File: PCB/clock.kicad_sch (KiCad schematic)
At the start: 22 parts, among them J1 USB_C_Receptacle, J2 Conn_01x08, J3 Conn_01x02_Pin, J4 Conn_01x05, J5 Conn_01x05, J6 Conn_01x08, J7 Conn_01x02_Pin, J8 Conn_01x05, J9 Conn_01x05, SW1 RotaryEncoder_Switch_MP, SW2 RotaryEncoder_Switch_MP, U1 ESP32-S3-MINI-1, U2 AMS1117-3.3

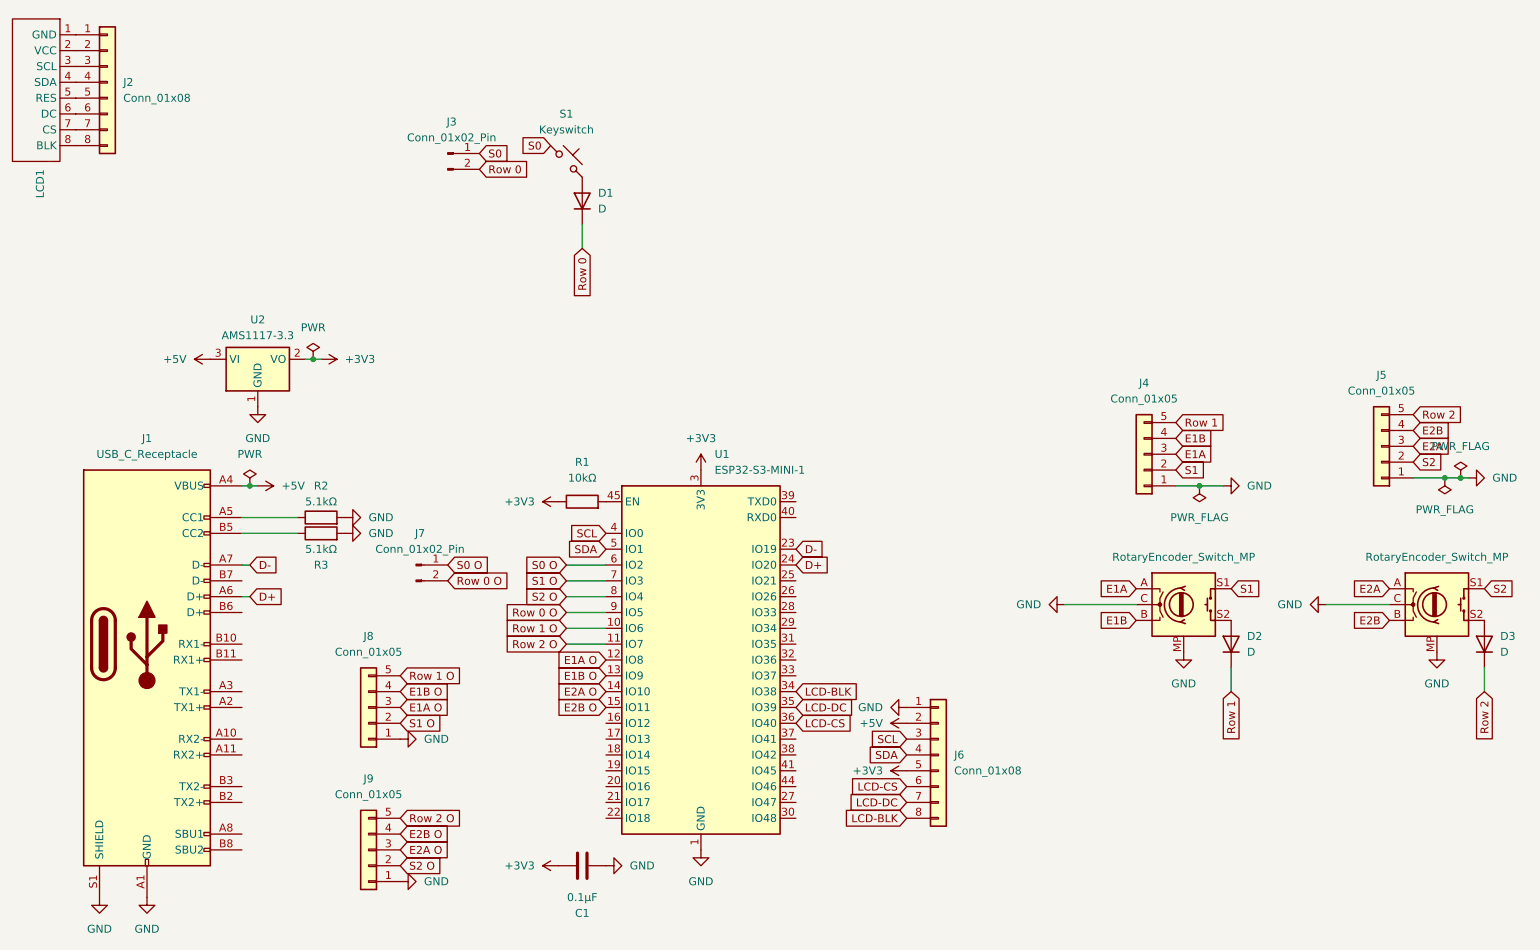
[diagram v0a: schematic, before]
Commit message: Add files via upload
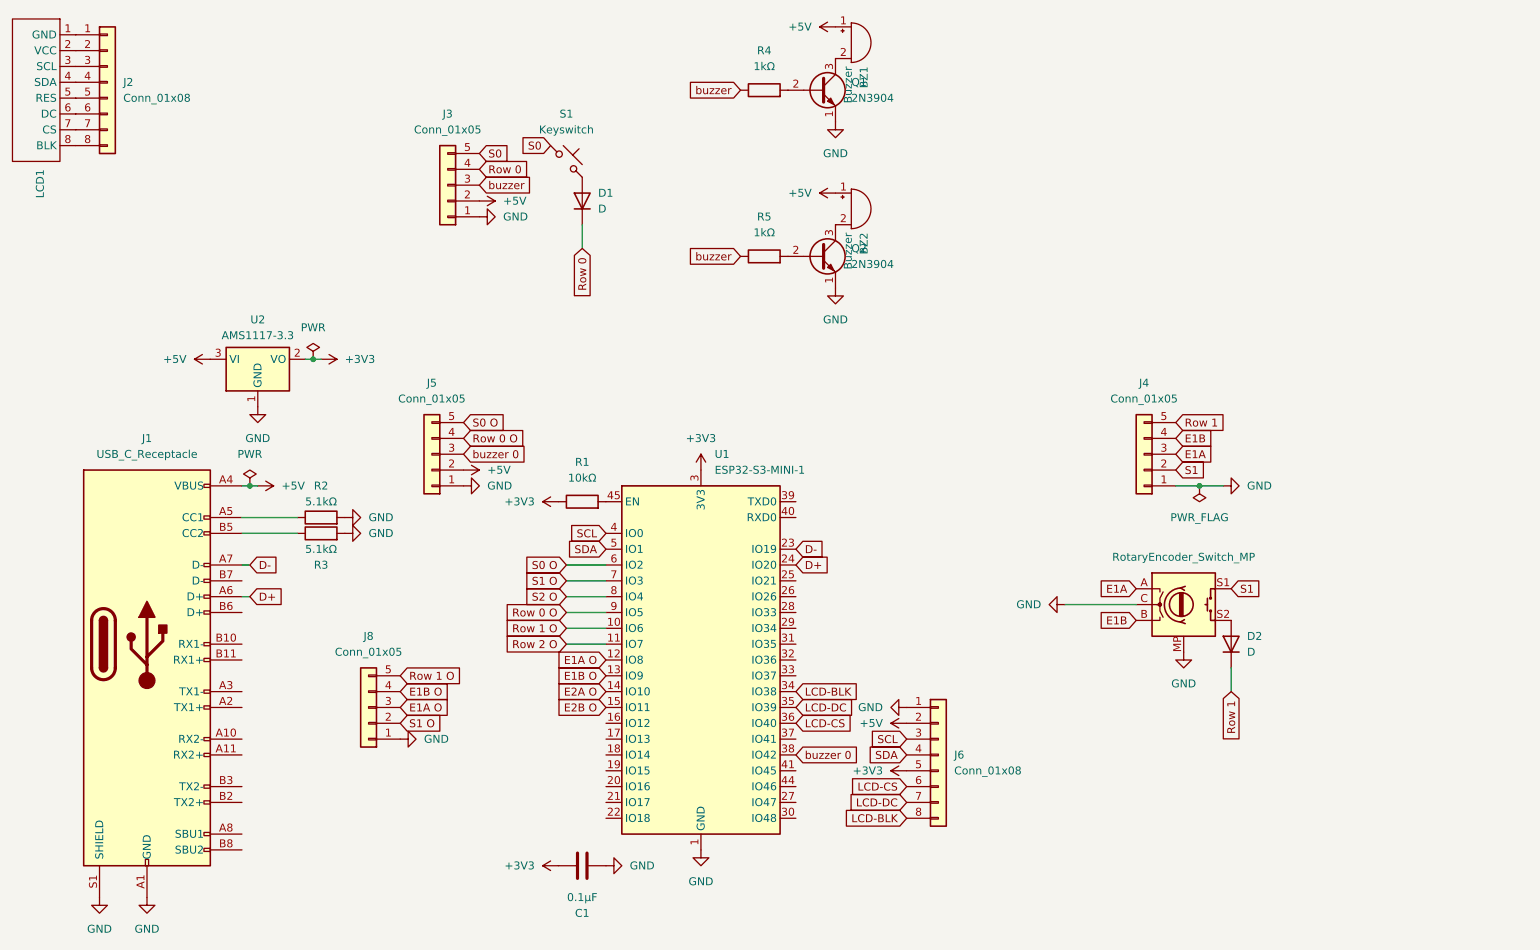
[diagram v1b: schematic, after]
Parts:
- removed D3: D, Diode_SMD:D_0603_1608Metric_Pad1.05x0.95mm_HandSolder, symbol Device:D
- removed J3, J7: Conn_01x02_Pin, Connector_JST:JST_XH_B2B-XH-A_1x02_P2.50mm_Vertical, symbol Connector:Conn_01x02_Pin
- removed J9: Conn_01x05, Connector_JST:JST_XH_B5B-XH-A_1x05_P2.50mm_Vertical, symbol Connector_Generic:Conn_01x05
- removed SW2: RotaryEncoder_Switch_MP, ScottoKeebs_Scotto:Encoder_EC11_MX, symbol Device:RotaryEncoder_Switch_MP
- added BZ1, BZ2: Buzzer, Buzzer_Beeper:Buzzer_12x9.5RM7.6, symbol Device:Buzzer
- added J3: Conn_01x05, Connector_JST:JST_XH_B5B-XH-A_1x05_P2.50mm_Vertical, symbol Connector_Generic:Conn_01x05
- added Q1, Q2: 2N3904, Package_TO_SOT_THT:TO-92_HandSolder, symbol Transistor_BJT:Q_NPN_EBC
- added R4, R5: 1kΩ, Capacitor_SMD:C_0603_1608Metric_Pad1.08x0.95mm_HandSolder, symbol Device:R
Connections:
- net E2A is gone; now on net buzzer 0: J5.3 (Pin_3)
- net E2B is gone; now on net Row 0 O: J5.4 (Pin_4)
- net Row 2 is gone; now on net S0 O: J5.5 (Pin_5)
- net S2 is gone; now on net +5V: J5.2 (Pin_2)
- net +5V: now also BZ1.1 (+), BZ2.1 (+), J3.2 (Pin_2)
- net GND: now also J3.1 (Pin_1), Q1.1 (E), Q2.1 (E)
- net Row 0: now also J3.4 (Pin_4)
- net S0: now also J3.5 (Pin_5)
- net buzzer 0: now reaches U1.38 (IO42)
- new net: Q1.2 (B), R4.2
- new net: BZ1.2 (-), Q1.3 (C)
- new net: BZ2.2 (-), Q2.3 (C)
- new net: Q2.2 (B), R5.2
- new net buzzer: J3.3 (Pin_3), R4.1, R5.1

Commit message: ready to submit?
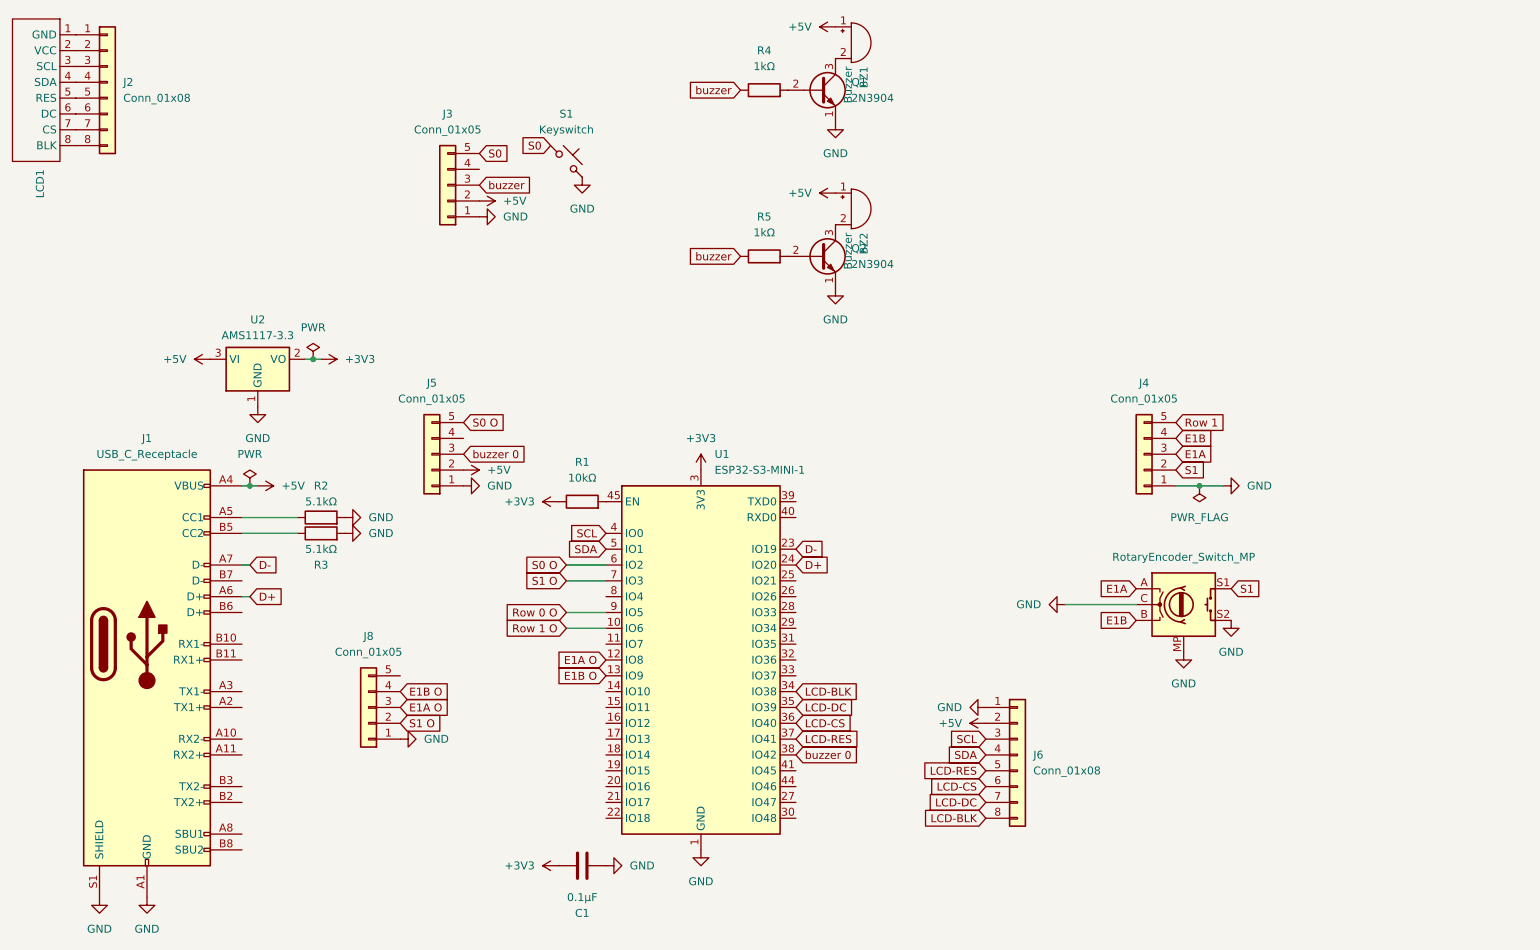
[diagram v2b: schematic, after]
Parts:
- removed D1, D2: D, Diode_SMD:D_0603_1608Metric_Pad1.05x0.95mm_HandSolder, symbol Device:D
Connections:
- net +3V3: no longer J6.5 (Pin_5)
- net GND: now also S1.2, SW1.S2
- net Row 0 O: no longer J5.4 (Pin_4)
- net Row 1 O: no longer J8.5 (Pin_5)
- net LCD-RES: now reaches U1.37 (IO41)
- net LCD-RES: now also J6.5 (Pin_5)
- net E2A O: no longer names the net of U1.14 (IO10)
- net E2B O: no longer names the net of U1.15 (IO11)
- net Row 0: no longer names the net of J3.4 (Pin_4)
- net Row 2 O: no longer names the net of U1.11 (IO7)
- net S2 O: no longer names the net of U1.8 (IO4)
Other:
- moved on the sheet: J6

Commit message: pcb remove hotswap switch
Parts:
- S1: footprint Gateron-low-profile:Gateron_Low_Profile_Socket_1U -> marbastlib-xp-gateron_lp:SW_KS33_1u
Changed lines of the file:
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@@
 			)
 		)
-		(property "Footprint" "Gateron-low-profile:Gateron_Low_Profile_Socket_1U"
+		(property "Footprint" "marbastlib-xp-gateron_lp:SW_KS33_1u"
 			(at 123.19 50.8 0)
 			(effects
